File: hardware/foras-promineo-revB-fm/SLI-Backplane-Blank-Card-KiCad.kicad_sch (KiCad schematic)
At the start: 25 parts, among them P1 Card Edge for HSEC8-160-01-S-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, Q10 MMBT3906-7-F, Q14 MMBT3906-7-F, Q205 MMBT4401-7-F, Q206 IRF7458, Q207 IRF7404, Q208 IRF7458, Q211 IRF7404, Q212 IRF7404, Q213 IRF7404, Q220 IRF7404, Q9 MMBT3906-7-F

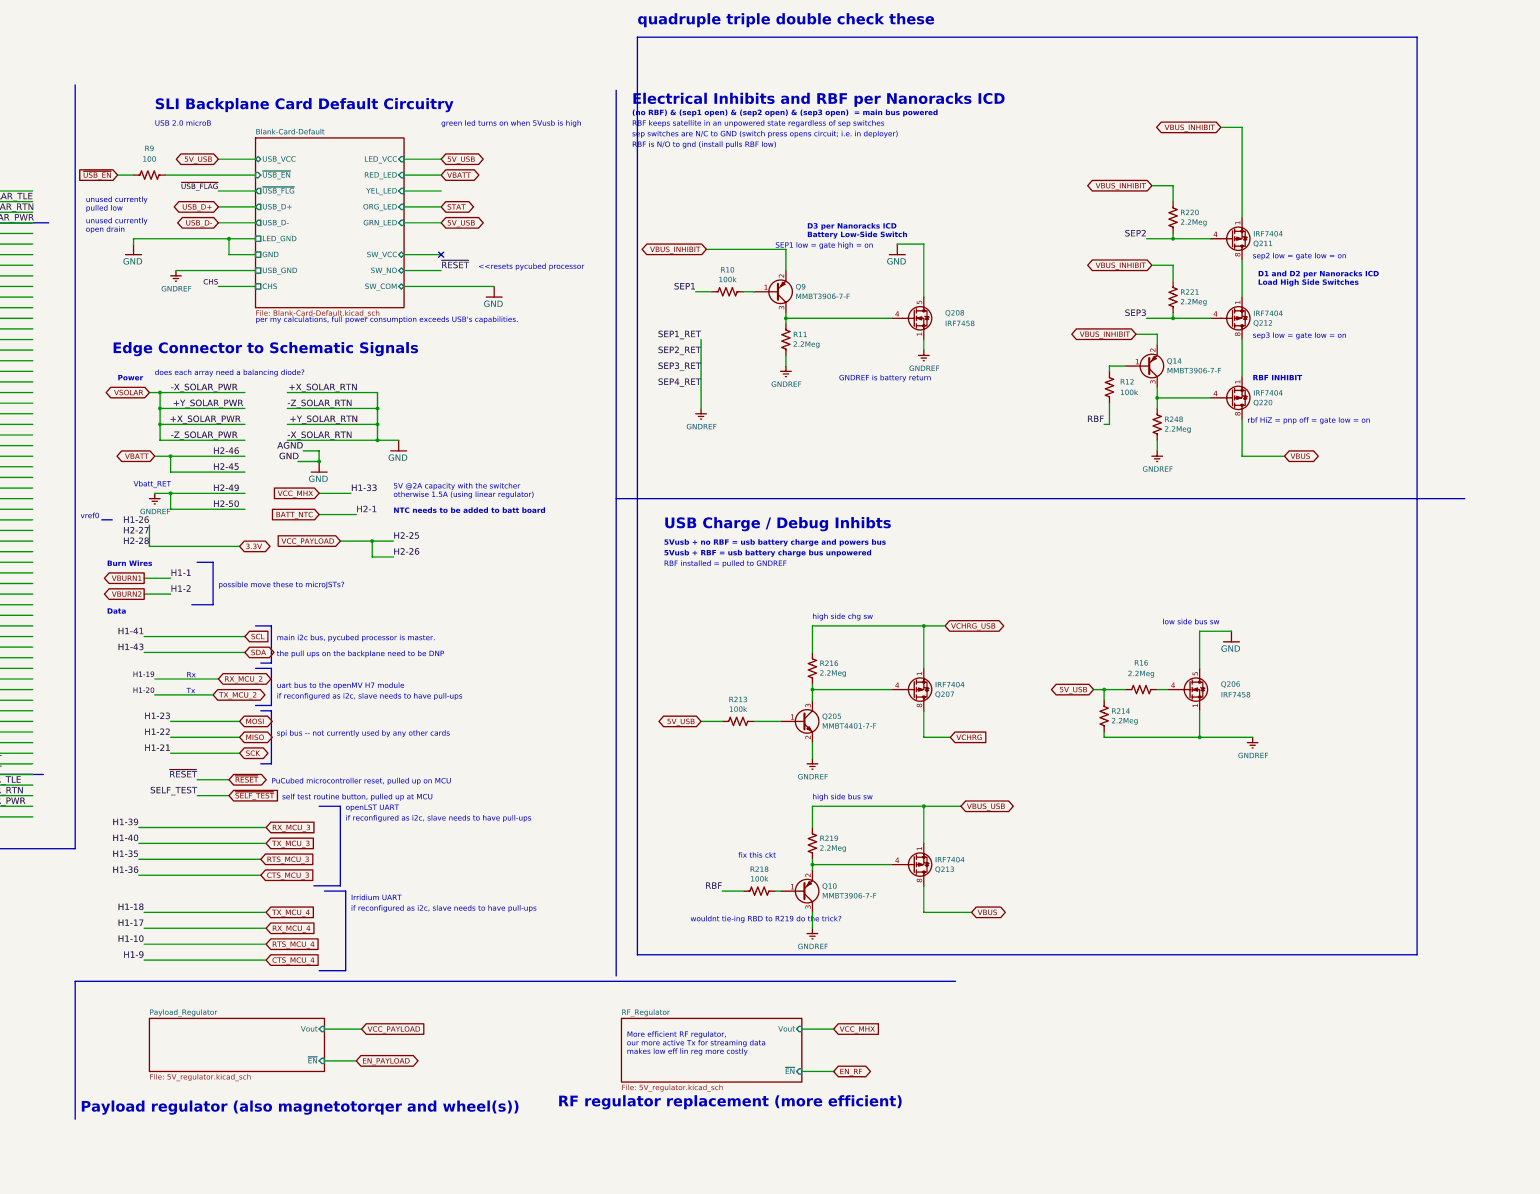
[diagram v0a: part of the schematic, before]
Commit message: fm sch changes
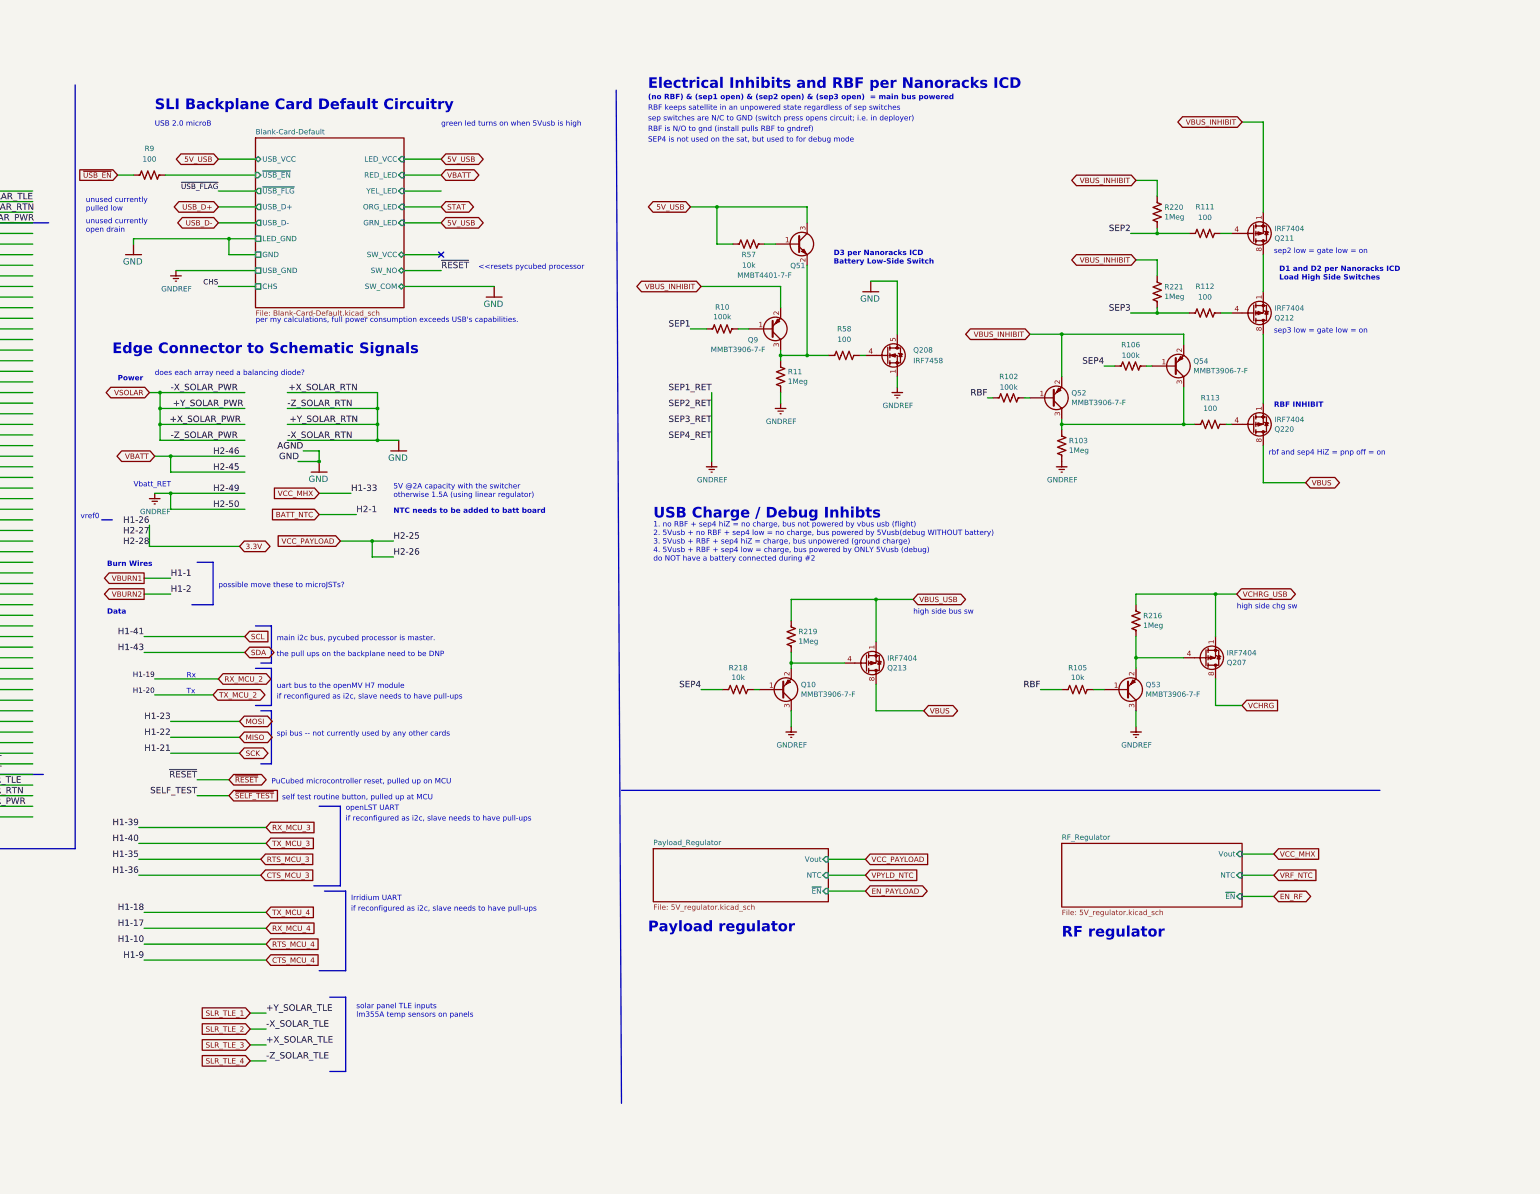
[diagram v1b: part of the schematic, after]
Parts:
- removed Q14: MMBT3906-7-F, Package_TO_SOT_SMD:SOT-23, symbol mainboard-rescue:Q_PNP_BEC-Device-mainboard-rescue
- removed Q205: MMBT4401-7-F, Package_TO_SOT_SMD:SOT-23, symbol mainboard-rescue:Q_NPN_BEC-Device-mainboard-rescue
- removed Q206: IRF7458, Package_SO:SOIC-8_3.9x4.9mm_P1.27mm, symbol mainboard_SLI:IRF7458
- removed R12: 100k, Resistor_SMD:R_0603_1608Metric, symbol Device:R_US
- removed R16: 2.2Meg, Resistor_SMD:R_0603_1608Metric, symbol Device:R_US
- removed R213: 100k, Resistor_SMD:R_0603_1608Metric, symbol mainboard-rescue:R_US-Device-mainboard-rescue
- removed R214, R248: 2.2Meg, Resistor_SMD:R_0603_1608Metric, symbol mainboard-rescue:R_US-Device-mainboard-rescue
- added Q51: MMBT4401-7-F, Package_TO_SOT_SMD:SOT-23, symbol mainboard-rescue:Q_NPN_BEC-Device-mainboard-rescue
- added Q52, Q53, Q54: MMBT3906-7-F, Package_TO_SOT_SMD:SOT-23, symbol mainboard-rescue:Q_PNP_BEC-Device-mainboard-rescue
- added R102, R106: 100k, Resistor_SMD:R_0603_1608Metric, symbol Device:R_US
- added R103: 1Meg, Resistor_SMD:R_0603_1608Metric, symbol Device:R_US
- added R105, R57: 10k, Resistor_SMD:R_0603_1608Metric, symbol Device:R_US
- added R111, R112, R113, R58: 100, Resistor_SMD:R_0603_1608Metric, symbol Device:R_US
- R10: symbol mainboard-rescue:R_US-Device-mainboard-rescue -> Device:R_US
- R11, R216, R219, R220, R221: value 2.2Meg -> 1Meg; symbol mainboard-rescue:R_US-Device-mainboard-rescue -> Device:R_US
- R218: value 100k -> 10k; symbol mainboard-rescue:R_US-Device-mainboard-rescue -> Device:R_US
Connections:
- net 5V_USB: now also Q51.3 (C), R57.2
- net GNDREF: now also Q53.3 (C), R103.2
- net RBF: now also R102.2, R105.2; no longer R218.2
- net SEP2: now also R111.1; no longer Q211.4 (G)
- net SEP3: now also R112.1; no longer Q212.4 (G)
- net SEP4: now also R218.2, R106.2
- net VBUS_INHIBIT: now also Q52.2 (E), Q54.2 (E)
- net at Q9.3 (C), R11.1: now also Q51.2 (E), R58.1; no longer Q208.4 (G)
- net at Q207.4 (G), R216.2: now also Q53.2 (E)
- net at Q220.4 (G): now also R113.2
- net +X_SOLAR_TLE renamed SLR_TLE_3
- net +Y_SOLAR_TLE renamed SLR_TLE_1
- net -X_SOLAR_TLE renamed SLR_TLE_2
- net -Z_SOLAR_TLE renamed SLR_TLE_4
- new net: Q208.4 (G), R58.2
- new net: Q211.4 (G), R111.2
- new net: Q212.4 (G), R112.2
- new net: Q52.1 (B), R102.1
- new net: Q52.3 (C), Q54.3 (C), R103.1, R113.1
- new net: Q54.1 (B), R106.1
- new net: Q53.1 (B), R105.1
- new net: Q51.1 (B), R57.1
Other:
- sheet Payload_Regulator ports: added NTC; removed none
- sheet RF_Regulator ports: added NTC; removed none
- note added: "1. no RBF + sep4 hiZ = no charge, bus not powered by vbus usb (flight) 2. 5Vusb + no RBF + sep4 low = no charge, bus powered by 5Vusb(debug WITHOUT battery) 3. 5Vusb + RBF + sep4 hiZ = charge, bus unpowered (ground charge) 4. 5Vusb + RBF + sep4 low = charge, bus powered by ONLY 5Vusb (debug) do NOT have a battery connected during #2"
- note added: "Payload regulator"
- note added: "RBF is N/O to gnd (install pulls RBF to gndref)"
- note added: "RF regulator"
- note added: "SEP4 is not used on the sat, but used to for debug mode"
- note added: "rbf and sep4 HiZ = pnp off = on"
- note added: "solar panel TLE inputs lm355A temp sensors on panels"
- note removed: "5Vusb + RBF = usb battery charge bus unpowered"
- note removed: "5Vusb + no RBF = usb battery charge and powers bus"
- note removed: "GNDREF is battery return"
- note removed: "More efficient RF regulator, our more active Tx for streaming data makes low eff lin reg more costly"
- note removed: "Payload regulator (also magnetotorqer and wheel(s))"
- note removed: "RBF installed = pulled to GNDREF"
- note removed: "RBF is N/O to gnd (install pulls RBF low)"
- note removed: "RF regulator replacement (more efficient)"
- note removed: "SEP1 low = gate high = on"
- note removed: "fix this ckt"
- note removed: "low side bus sw"
- note removed: "quadruple triple double check these"
- note removed: "rbf HiZ = pnp off = gate low = on"
- note removed: "wouldnt tie-ing RBD to R219 do the trick?"
- moved on the sheet: Q10, Q207, Q208, Q211, Q212, Q213, Q220, Q9, R10, R11, R216, R218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
